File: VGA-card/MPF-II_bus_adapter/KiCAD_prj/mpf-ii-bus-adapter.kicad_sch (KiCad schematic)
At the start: 34 parts, among them J1 Bus_Apple_II_Card_Side, J10 USER1_Sel, J11 INH_Sel, J12 RDY_Sel, J13 COLREF_Sel, J14 IOSTRB_Sel, J15 Q3_Sel, J16 Pin, J17 Pin, J18 Pin, J19 Pin, J2 Bus_Apple_II_Computer_Side, J20 Pin, J21 Pin, J22 Pin, J23 Pin, J24 Pin, J25 Pin, J26 7M_Sel, J27 PWR, J3 DevSel_Sel, J4 Phi0_Sel, J5 Conn_02x25_Odd_Even, J6 SYNC_Sel, J7 DMA_Sel, J8 IRQ_Sel, J9 NMI_Sel, U1 74LS04

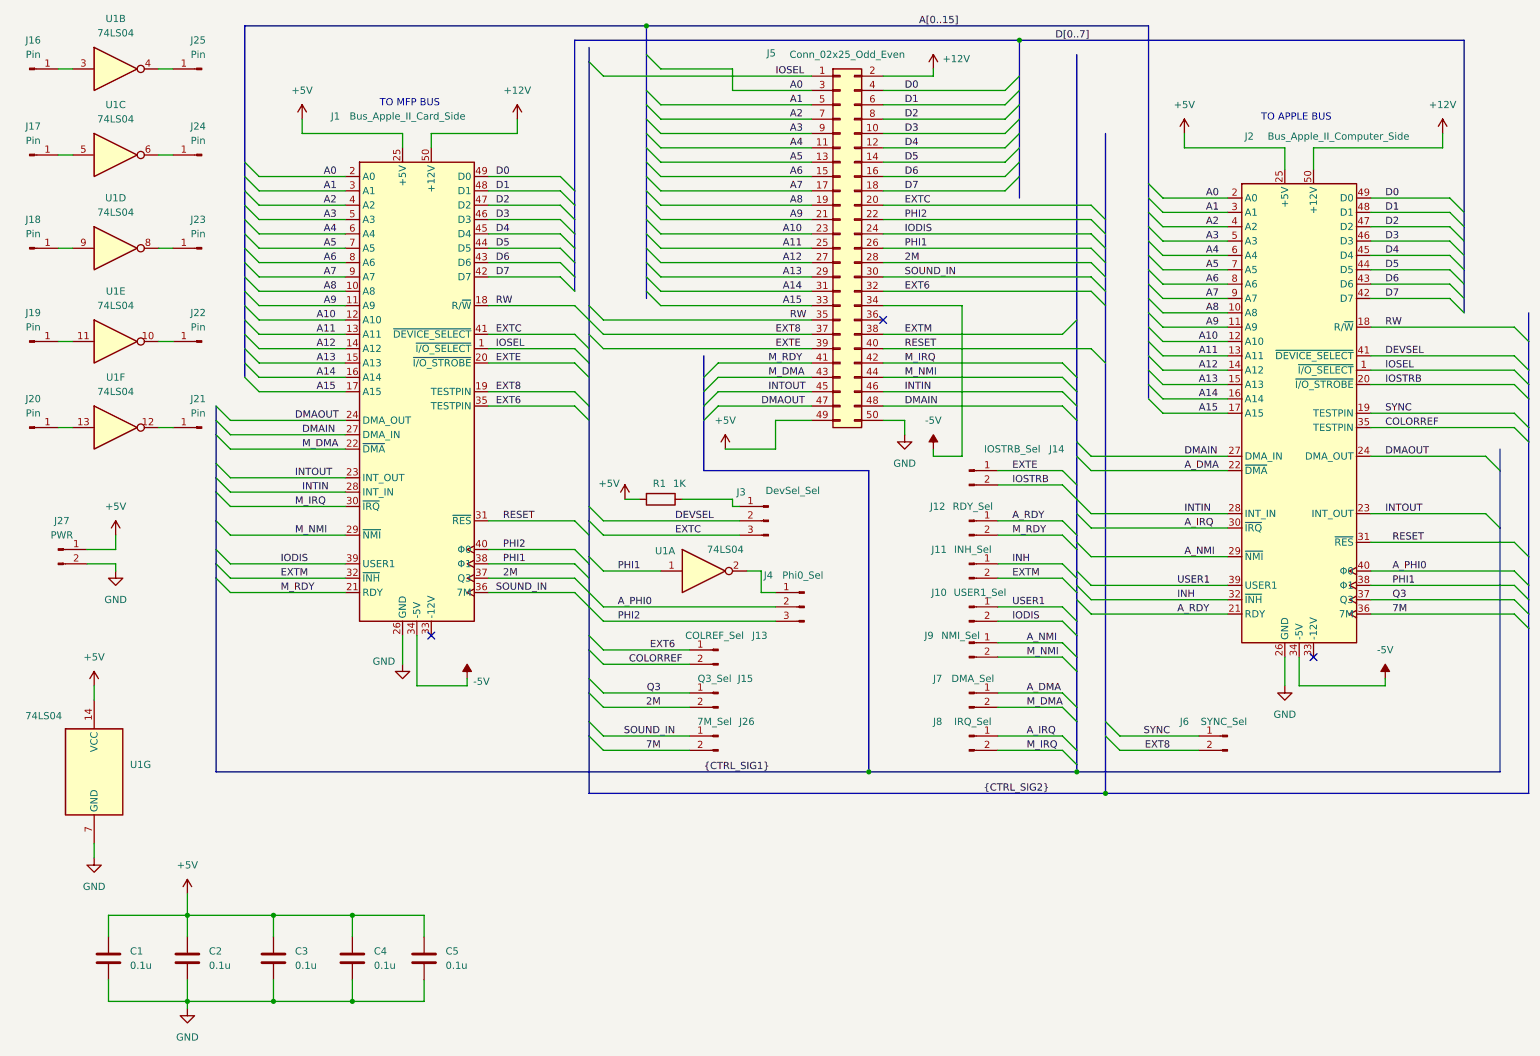
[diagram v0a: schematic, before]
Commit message: PCB
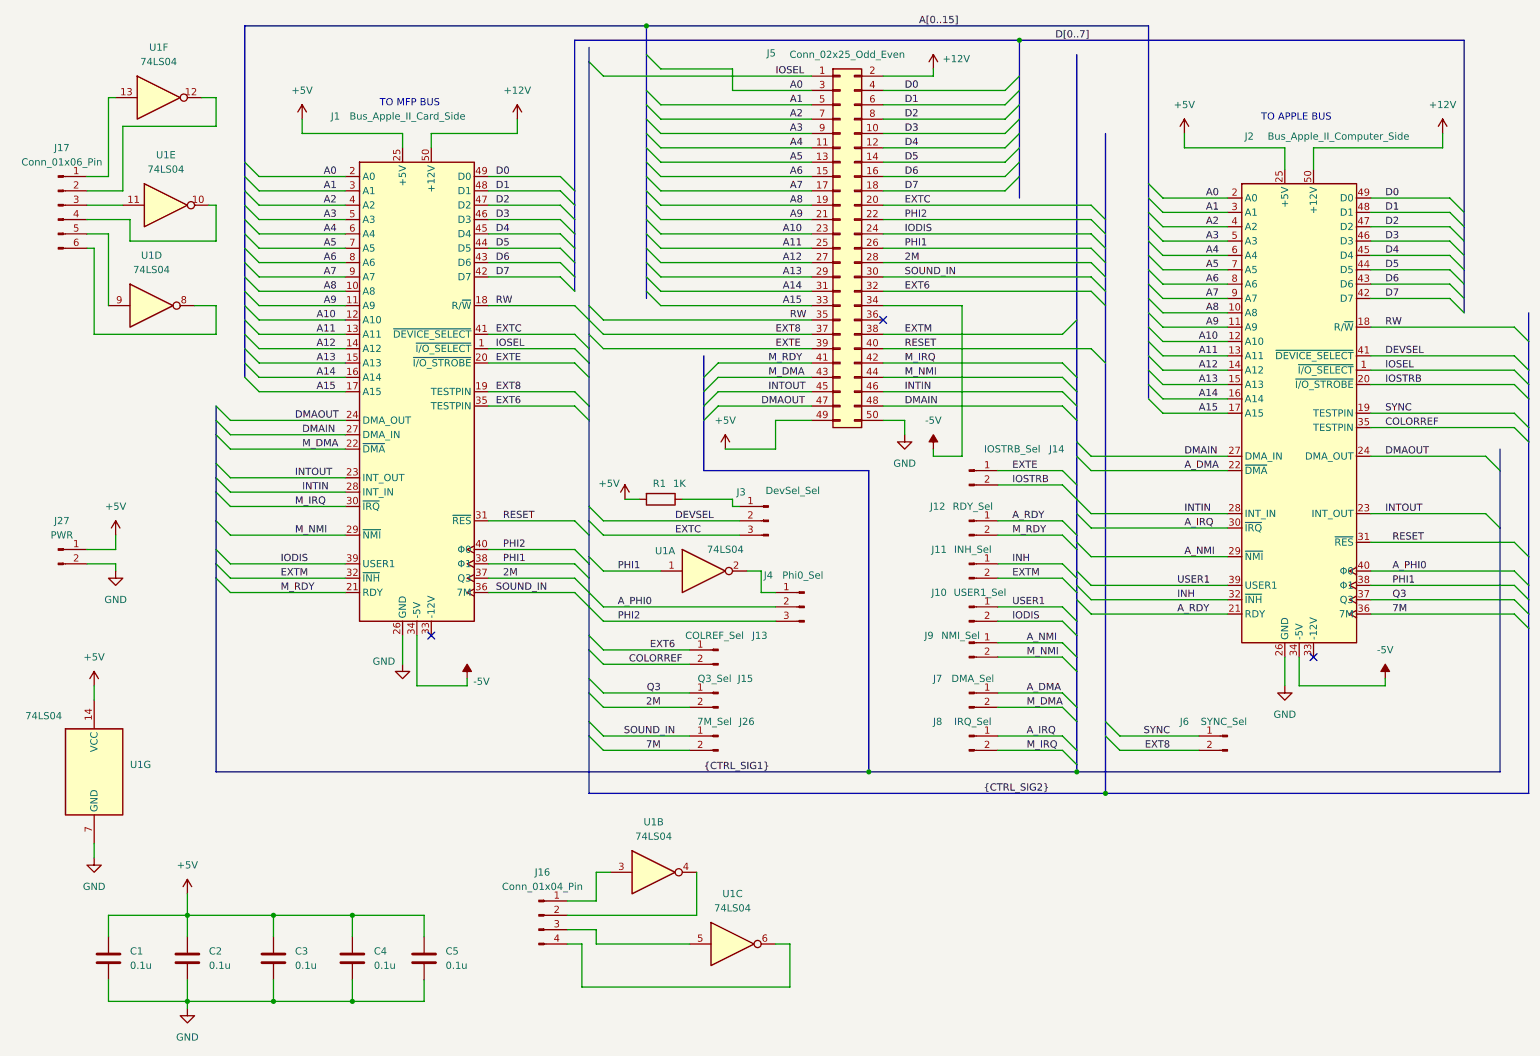
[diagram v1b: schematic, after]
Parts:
- removed J16, J17, J18, J19, J20, J21, J22, J23, J24, J25: Pin, Connector_PinHeader_2.00mm:PinHeader_1x01_P2.00mm_Vertical, symbol Connector:Conn_01x01_Pin
- added J16: Conn_01x04_Pin, Connector_PinHeader_2.54mm:PinHeader_1x04_P2.54mm_Vertical, symbol Connector:Conn_01x04_Pin
- added J17: Conn_01x06_Pin, Connector_PinHeader_2.54mm:PinHeader_1x06_P2.54mm_Vertical, symbol Connector:Conn_01x06_Pin
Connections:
- net at U1.9: now also J17.5 (Pin_5)
- net at U1.3: now also J16.1 (Pin_1)
- net at U1.11: now also J17.3 (Pin_3)
- net at U1.10: now also J17.4 (Pin_4)
- net at U1.5: now also J16.3 (Pin_3)
- net at U1.6: now also J16.4 (Pin_4)
- net at U1.12: now also J17.2 (Pin_2)
- net at U1.13: now also J17.1 (Pin_1)
- net at U1.8: now also J17.6 (Pin_6)
- net at U1.4: now also J16.2 (Pin_2)
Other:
- moved on the sheet: U1B, U1C, U1D, U1E, U1F
